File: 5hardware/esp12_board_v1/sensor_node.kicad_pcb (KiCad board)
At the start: 2 copper layers, 24.7 x 24.7 mm, 15 parts, among them J1 Conn_01x09_Pin, J2 Conn_01x06_Pin, SW2 SW_Push, SW7 SW_Push, U1 ESP-12F

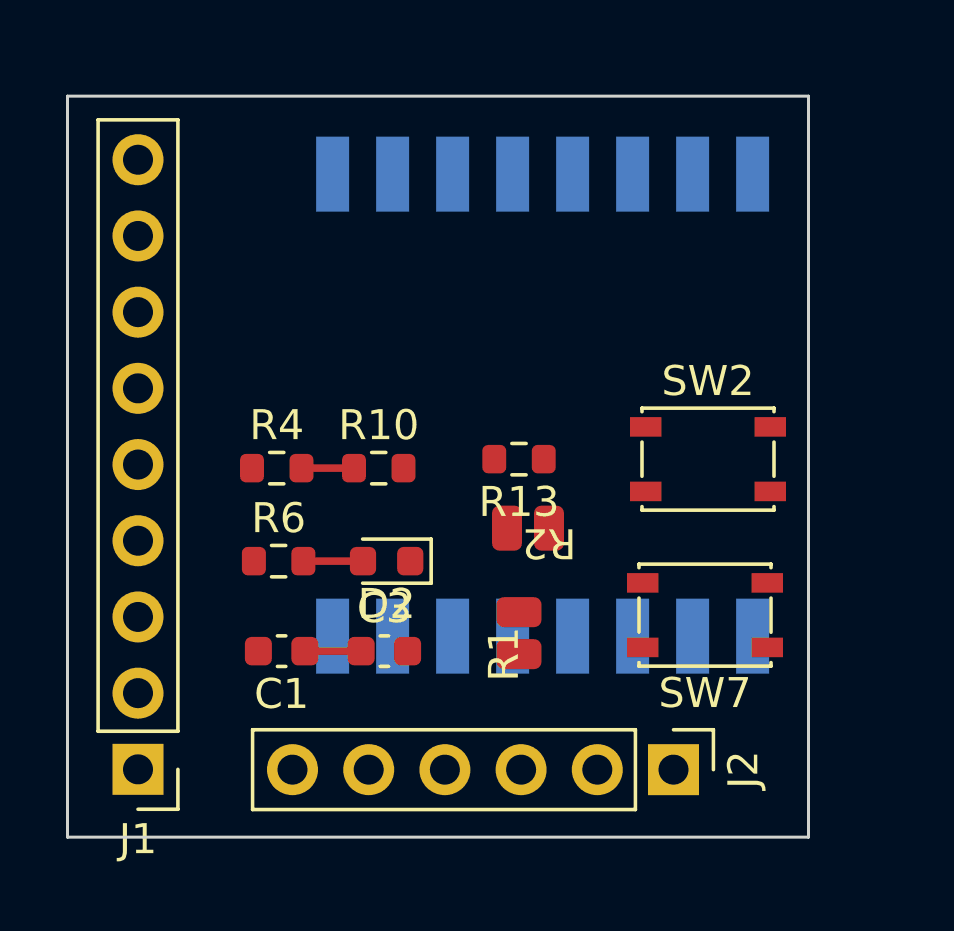
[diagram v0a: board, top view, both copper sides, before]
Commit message: update PCBs.
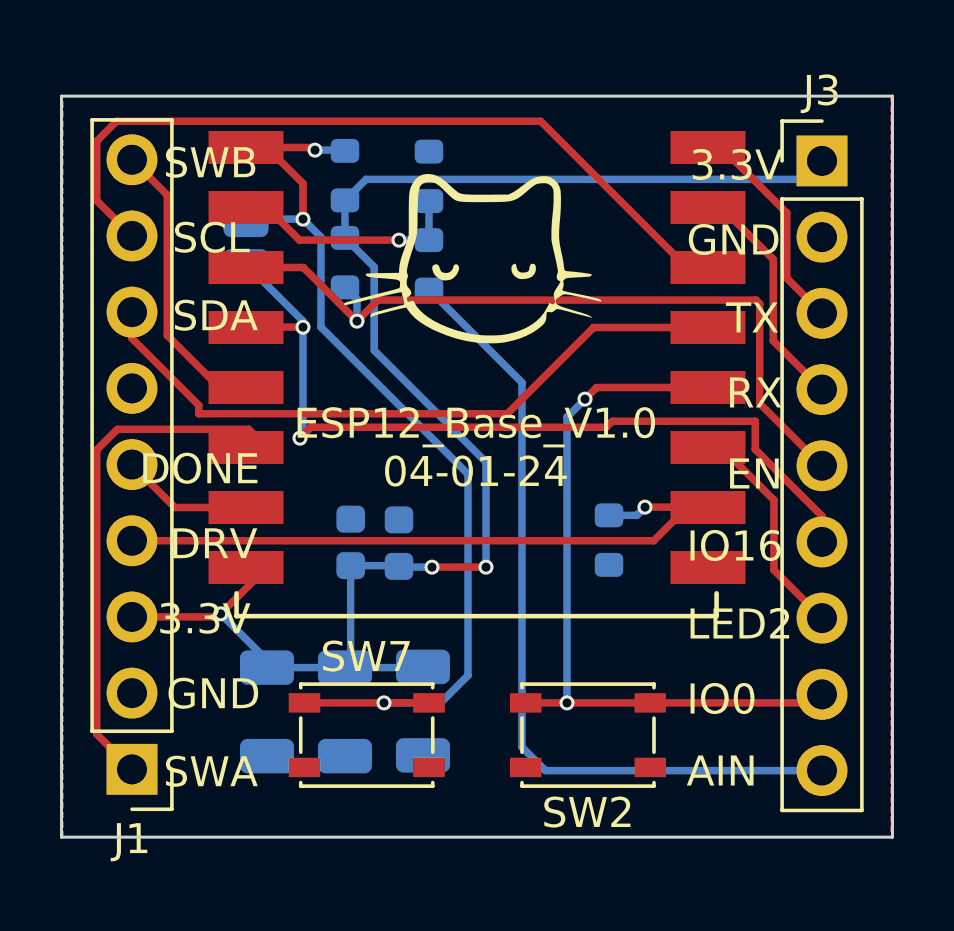
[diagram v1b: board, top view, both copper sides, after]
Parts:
- removed D2: LED, LED_SMD:LED_0603_1608Metric
- removed J2: Conn_01x06_Pin, Connector_PinHeader_2.54mm:PinHeader_1x06_P2.54mm_Vertical
- removed R6: R, Resistor_SMD:R_0603_1608Metric
- added C2: 100u, Capacitor_SMD:C_1206_3216Metric, B.Cu at (147.4, 78.9)
- added C4: 10u, Capacitor_SMD:C_0603_1608Metric, B.Cu at (146.6, 73.3)
- added C5: .1u, Capacitor_SMD:C_0603_1608Metric, B.Cu at (145.0, 73.3)
- added J3: Conn_01x09_Pin, Connector_PinHeader_2.54mm:PinHeader_1x09_P2.54mm_Vertical, F.Cu at (160.7, 60.6)
- added R3: R, Resistor_SMD:R_0603_1608Metric, B.Cu at (147.6, 61.1)
- C1, C3: value C -> 100u; footprint Capacitor_SMD:C_0603_1608Metric -> Capacitor_SMD:C_1206_3216Metric; moved to B.Cu
- G***, U1: moved to F.Cu
- R1: footprint A_SensorNode:Jumpper -> Resistor_SMD:R_0603_1608Metric; moved to B.Cu
- R10, R13, R2, R4: moved to B.Cu
- moved U1 27.6 mm to (141.2, 57.5), turned to 0 degrees
- moved R2 13.4 mm to (141.5, 64.0), turned to 90 degrees
- moved R1 13.3 mm to (147.6, 64.0), turned to -90 degrees
- moved SW7 12.0 mm to (145.5, 79.7), turned to 0 degrees
- moved SW2 10.0 mm to (152.9, 79.7), turned to 180 degrees
- moved R4 10.0 mm to (144.8, 61.0), turned to -90 degrees
- moved R10 6.94 mm to (144.8, 63.9), turned to -90 degrees
- moved G*** 5.80 mm to (149.2, 63.8), turned to 0 degrees
- moved R13 4.04 mm to (153.6, 73.2), turned to 90 degrees
- moved C3 2.41 mm to (144.8, 78.9), turned to -90 degrees
- moved C1 2.08 mm to (142.2, 78.9), turned to -90 degrees
- moved J1 0.20 mm to (137.7, 80.8)
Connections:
- net Net-(U1-GPIO0) renamed IO0
- R1 pad 1: Net-(D2-K) -> ADC
- R1 pad 2: GND -> Net-(J3-Pin_9)
- U1 pad 2: unconnected-(U1-ADC-Pad2) -> ADC
- U1 pad 5: SW-A -> SW-B
- U1 pad 6: SW-B -> SW-A
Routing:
- net +3.3V: track 3.72 -> 51.5 mm, vias 0 -> 3
- net Net-(U1-REST): track 0.00 -> 32.3 mm, vias 0 -> 3
- net IO16: track 0.00 -> 28.2 mm, vias 0 -> 2
- net Net-(J3-Pin_9): track 0.00 -> 26.9 mm
- net SCL: track 0.00 -> 25.6 mm
- net EN: track 0.00 -> 25.1 mm, vias 0 -> 1
- net IO0: track 0.00 -> 23.9 mm, vias 0 -> 2
- net SDA: track 0.00 -> 21.8 mm
- net DRIVE: track 0.00 -> 21.7 mm, vias 0 -> 1
- net SW-A: track 0.00 -> 17.3 mm
- net SW-B: track 0.00 -> 10.4 mm
- net RX: track 0.00 -> 8.61 mm
- net LED2: track 0.00 -> 8.23 mm
- net TX: track 0.00 -> 8.07 mm
- net ADC: track 0.00 -> 7.15 mm, vias 0 -> 1
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- added copper zone on B.Cu, net GND
- added copper zone on F.Cu, net GND
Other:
- board size 24.7 x 24.7 mm -> 27.7 x 24.7 mm
- board text added: "3.3V"
- board text added: "AIN"
- board text added: "DONE"
- board text added: "DRV"
- board text added: "EN"
- board text added: "ESP12_Base_V1.0 04-01-24"
- board text added: "GND"
- board text added: "IO0"
- board text added: "IO16"
- board text added: "LED2"
- board text added: "RX"
- board text added: "SCL"
- board text added: "SDA"
- board text added: "SWA"
- board text added: "SWB"
- board text added: "TX"
- board text removed: "ESP-MESS B V13.2"
